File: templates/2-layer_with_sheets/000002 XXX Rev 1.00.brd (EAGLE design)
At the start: 130 x 230 mm, 21 parts, among them X1 PAD_TEST_GROUND_HOOK

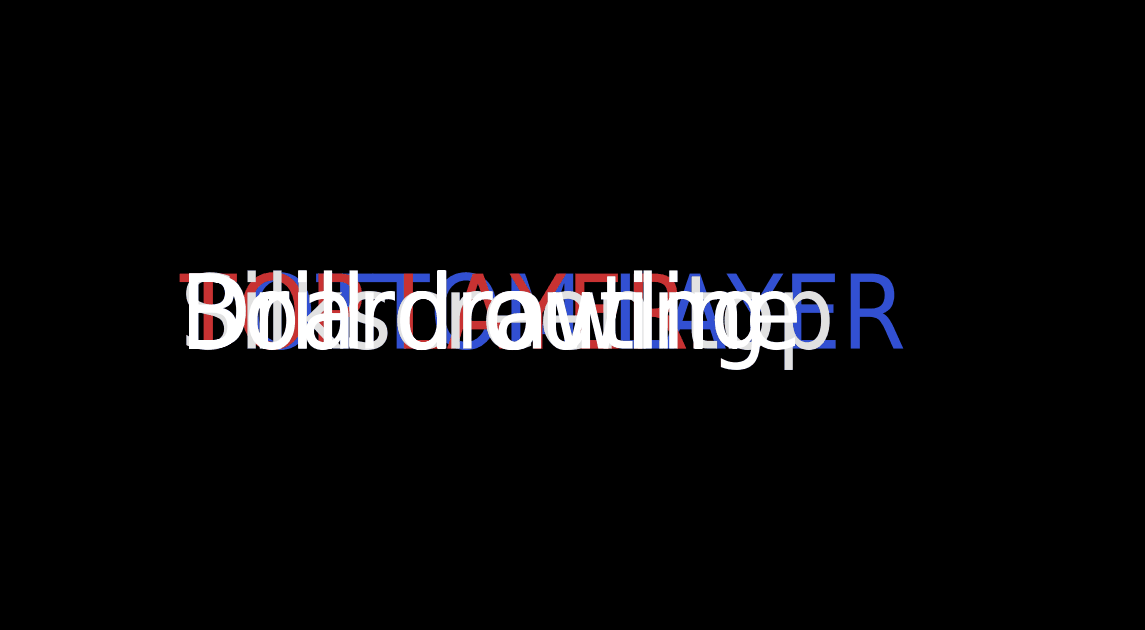
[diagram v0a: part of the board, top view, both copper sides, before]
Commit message: bugfixes
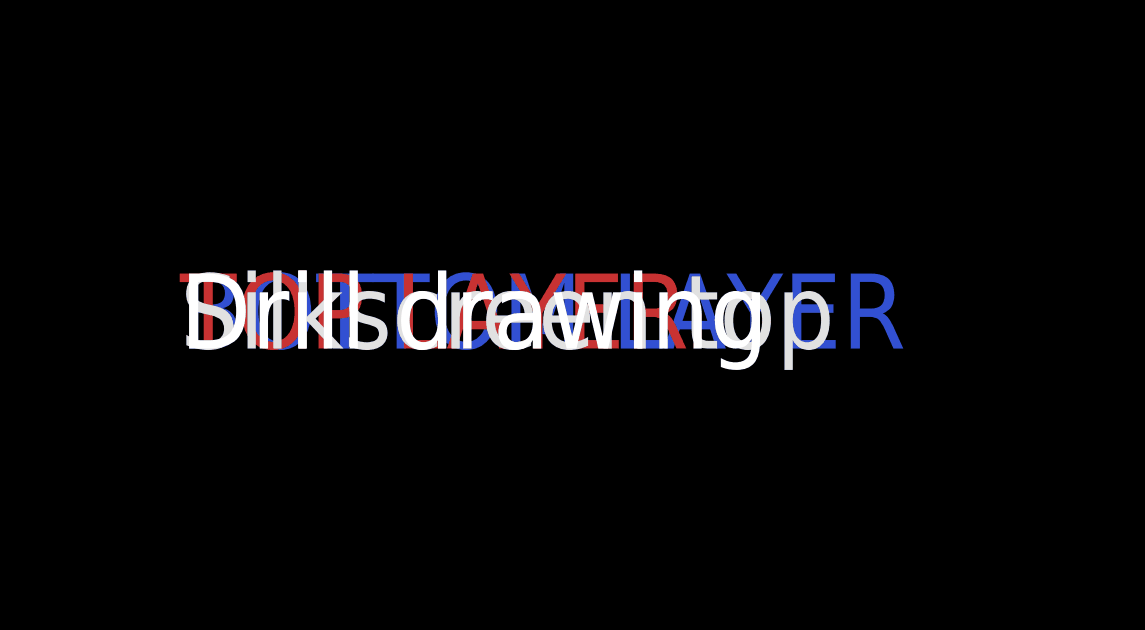
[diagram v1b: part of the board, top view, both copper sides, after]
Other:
- board text removed: "Board outline"
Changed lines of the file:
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@@
 <text x="101" y="210" size="2.5" layer="46" font="vector" ratio="12" align="top-left">Order form</text>
 <text x="101" y="204" size="2.5" layer="46" font="vector" ratio="12" align="top-left">Order form</text>
-<text x="134" y="26" size="2.5" layer="20" font="vector" ratio="12" align="top-left">Board outline</text>
 </plain>
 <attributes>
